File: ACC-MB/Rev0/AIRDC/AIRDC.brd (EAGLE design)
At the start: 70 x 75 mm, 4 parts

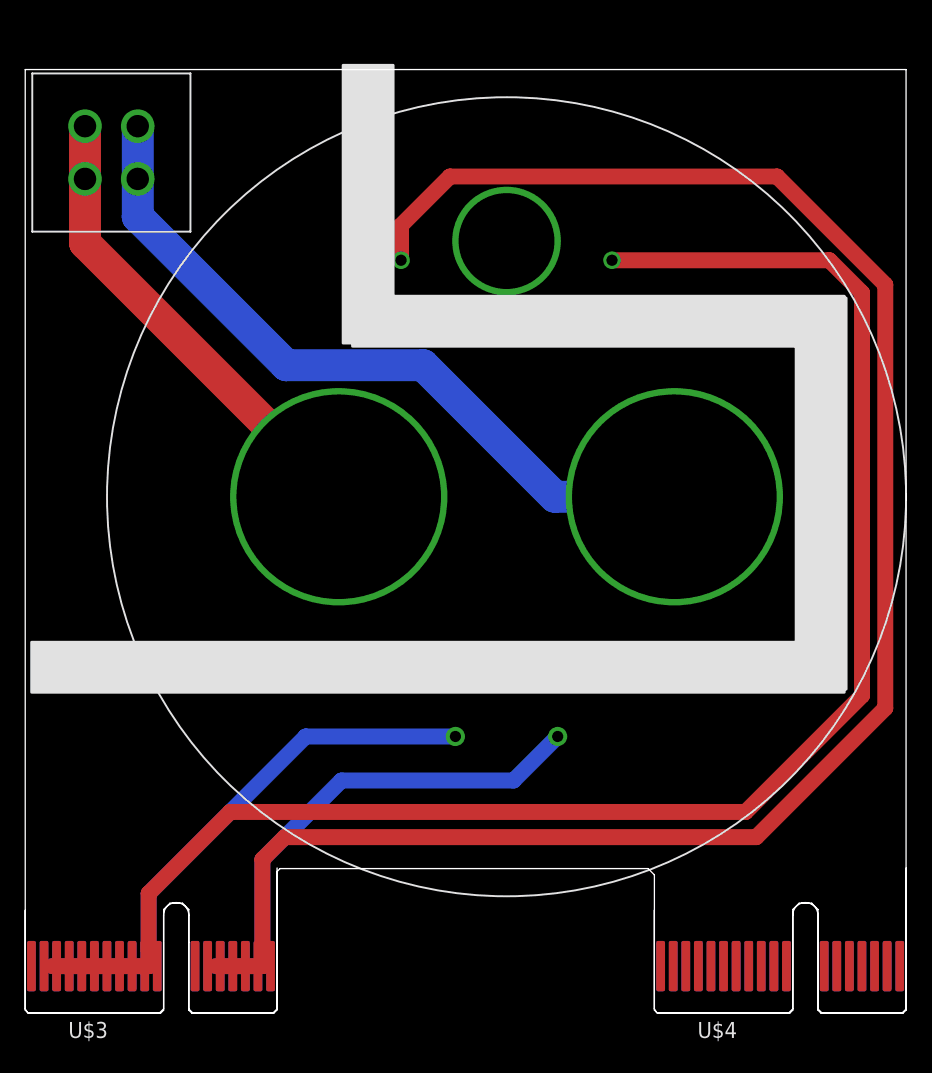
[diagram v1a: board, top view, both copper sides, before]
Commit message: update
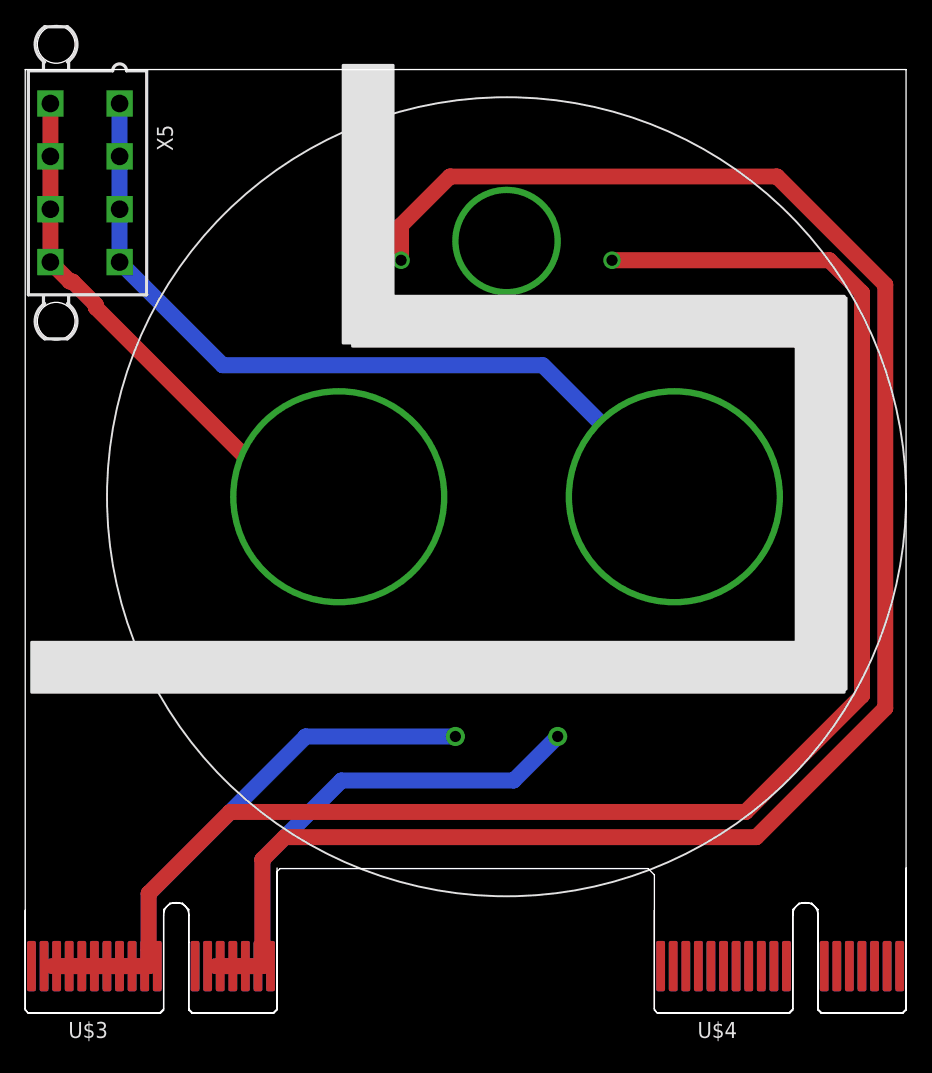
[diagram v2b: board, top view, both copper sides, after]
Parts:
- removed U$2: IPBT-102-H1-T-D, ACC-MB-R0:IPBT-102-H1-T-D
- added X5: 5566-8, con-molex:5566-8
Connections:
- removed net N$8: U$1.A2, U$2.P$3, U$2.P$4
- new net N$5: U$1.A1, X5.5, X5.6, X5.7, X5.8
- net N$6: now also U$1.A2, X5.1, X5.2, X5.3, X5.4; no longer U$1.A1, U$2.P$1, U$2.P$2
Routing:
- net N$8: track 59.1 -> 0.00 mm
- net N$5: track 0.00 -> 43.4 mm
- net N$6: track 37.8 -> 64.4 mm
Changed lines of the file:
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@@
 <drawing>
 <settings>
-<setting alwaysvectorfont="yes"/>
+<setting alwaysvectorfont="no"/>
 <setting verticaltext="up"/>
 </settings>
@@
 <elements>
 <element name="U$1" library="ACC-MB-R0" library_urn="urn:adsk.eagle:library:13324935" package="GV224" package3d_urn="urn:adsk.eagle:package:13209922/2" value="GV224" x="38" y="22"/>
-<element name="U$2" library="ACC-MB-R0" library_urn="urn:adsk.eagle:library:13324935" package="IPBT-102-H1-T-D" package3d_urn="urn:adsk.eagle:package:13324986/2" value="IPBT-102-H1-T-D" x="4.5" y="70.5" rot="R270"/>
 <element name="U$3" library="ACC-MB-R0" library_urn="urn:adsk.eagle:library:13324935" package="PCI-E_SLOT_36" value="PCIE-36-EDGE" x="0" y="0"/>
 <element name="U$4" library="ACC-MB-R0" library_urn="urn:adsk.eagle:library:13324935" package="PCI-E_SLOT_36" value="PCIE-36-EDGE" x="50" y="0"/>
+<element name="X5" library="con-molex" library_urn="urn:adsk.eagle:library:165" package="5566-8" value="5566-8" x="4.5" y="66" rot="R90">
+<attribute name="MF" value="MOLEX" x="4.5" y="66" size="1.778" layer="27" rot="R90" display="off"/>
+<attribute name="MPN" value="" x="4.5" y="66" size="1.778" layer="27" rot="R90" display="off"/>
+<attribute name="OC_FARNELL" value="unknown" x="4.5" y="66" size="1.778" layer="27" rot="R90" display="off"/>
+<attribute name="OC_NEWARK" value="unknown" x="4.5" y="66" size="1.778" layer="27" rot="R90" display="off"/>
+</element>
 </elements>
 <signals>
@@
 <wire x1="4.245" y1="3.75" x2="5.245" y2="3.75" width="0" layer="19" extent="16-16"/>
 <wire x1="0.245" y1="3.75" x2="1.245" y2="3.75" width="0" layer="19" extent="16-16"/>
-</signal>
-<signal name="N$6">
-<contactref element="U$1" pad="A1"/>
-<contactref element="U$2" pad="P$1"/>
-<contactref element="U$2" pad="P$2"/>
-<wire x1="4.5" y1="70.5" x2="4.5" y2="66.31" width="2.54" layer="1"/>
-<wire x1="4.5" y1="66.31" x2="4.5" y2="61.215" width="2.54" layer="1"/>
-<wire x1="4.5" y1="61.215" x2="24.665" y2="41.05" width="2.54" layer="1"/>
-</signal>
-<signal name="N$8">
-<contactref element="U$1" pad="A2"/>
-<contactref element="U$2" pad="P$3"/>
-<contactref element="U$2" pad="P$4"/>
-<wire x1="8.69" y1="70.5" x2="8.69" y2="66.31" width="2.54" layer="16"/>
-<wire x1="8.69" y1="66.31" x2="8.69" y2="63.31" width="2.54" layer="16"/>
-<wire x1="31.385" y1="51.5" x2="41.835" y2="41.05" width="2.54" layer="16"/>
-<wire x1="8.69" y1="63.31" x2="20.5" y2="51.5" width="2.54" layer="16"/>
-<wire x1="20.5" y1="51.5" x2="31.385" y2="51.5" width="2.54" layer="16"/>
-<wire x1="41.835" y1="41.05" x2="51.335" y2="41.05" width="2.54" layer="16"/>
 </signal>
 <signal name="N$1">
@@
 <wire x1="13.245" y1="3.75" x2="14.245" y2="3.75" width="0" layer="19" extent="16-16"/>
 </signal>
+<signal name="N$5">
+<contactref element="U$1" pad="A1"/>
+<contactref element="X5" pad="5"/>
+<contactref element="X5" pad="6"/>
+<contactref element="X5" pad="7"/>
+<contactref element="X5" pad="8"/>
+<wire x1="24.665" y1="41.05" x2="20.4" y2="41.05" width="1.27" layer="1"/>
+<wire x1="20.4" y1="41.05" x2="5.36100625" y2="56.08899375" width="1.27" layer="1"/>
+<wire x1="5.36100625" y1="56.08899375" x2="5.36100625" y2="56.3051875" width="1.27" layer="1"/>
+<wire x1="5.36100625" y1="56.3051875" x2="3.51519375" y2="58.151" width="1.27" layer="1"/>
+<wire x1="3.51519375" y1="58.151" x2="3.299" y2="58.151" width="1.27" layer="1"/>
+<wire x1="3.299" y1="58.151" x2="1.75" y2="59.7" width="1.27" layer="1"/>
+<wire x1="1.75" y1="59.7" x2="1.75" y2="63.9" width="1.27" layer="1"/>
+<wire x1="1.75" y1="63.9" x2="1.75" y2="68.1" width="1.27" layer="1"/>
+<wire x1="1.75" y1="68.1" x2="1.75" y2="72.3" width="1.27" layer="1"/>
+</signal>
+<signal name="N$6">
+<contactref element="X5" pad="1"/>
+<contactref element="X5" pad="2"/>
+<contactref element="X5" pad="3"/>
+<contactref element="X5" pad="4"/>
+<contactref element="U$1" pad="A2"/>
+<wire x1="51.335" y1="41.05" x2="40.885" y2="51.5" width="1.27" layer="16"/>
+<wire x1="15.45" y1="51.5" x2="7.25" y2="59.7" width="1.27" layer="16"/>
+<wire x1="40.885" y1="51.5" x2="15.45" y2="51.5" width="1.27" layer="16"/>
+<wire x1="7.25" y1="59.7" x2="7.25" y2="63.9" width="1.27" layer="16"/>
+<wire x1="7.25" y1="63.9" x2="7.25" y2="68.1" width="1.27" layer="16"/>
+<wire x1="7.25" y1="68.1" x2="7.25" y2="72.3" width="1.27" layer="16"/>
+</signal>
 </signals>
